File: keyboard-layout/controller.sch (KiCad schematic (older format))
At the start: 15 parts, among them J1 USB_mini_micro_B, SW1 SW_PUSH, X1 XTAL_GND

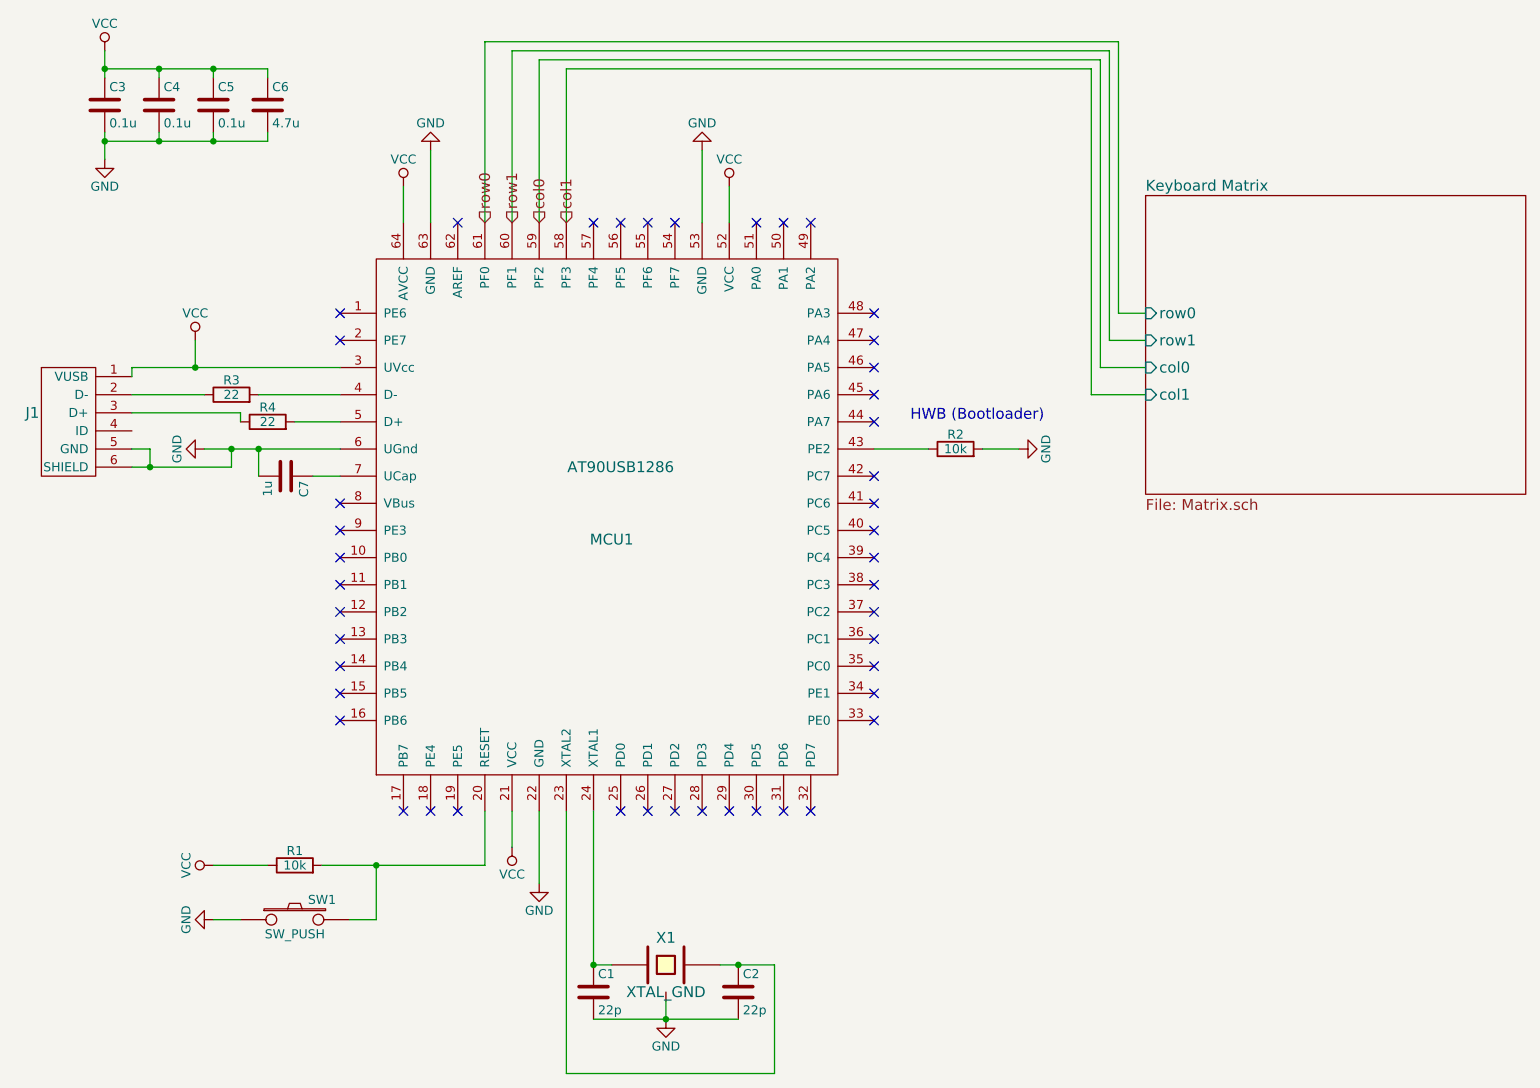
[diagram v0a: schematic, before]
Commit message: mx footprints
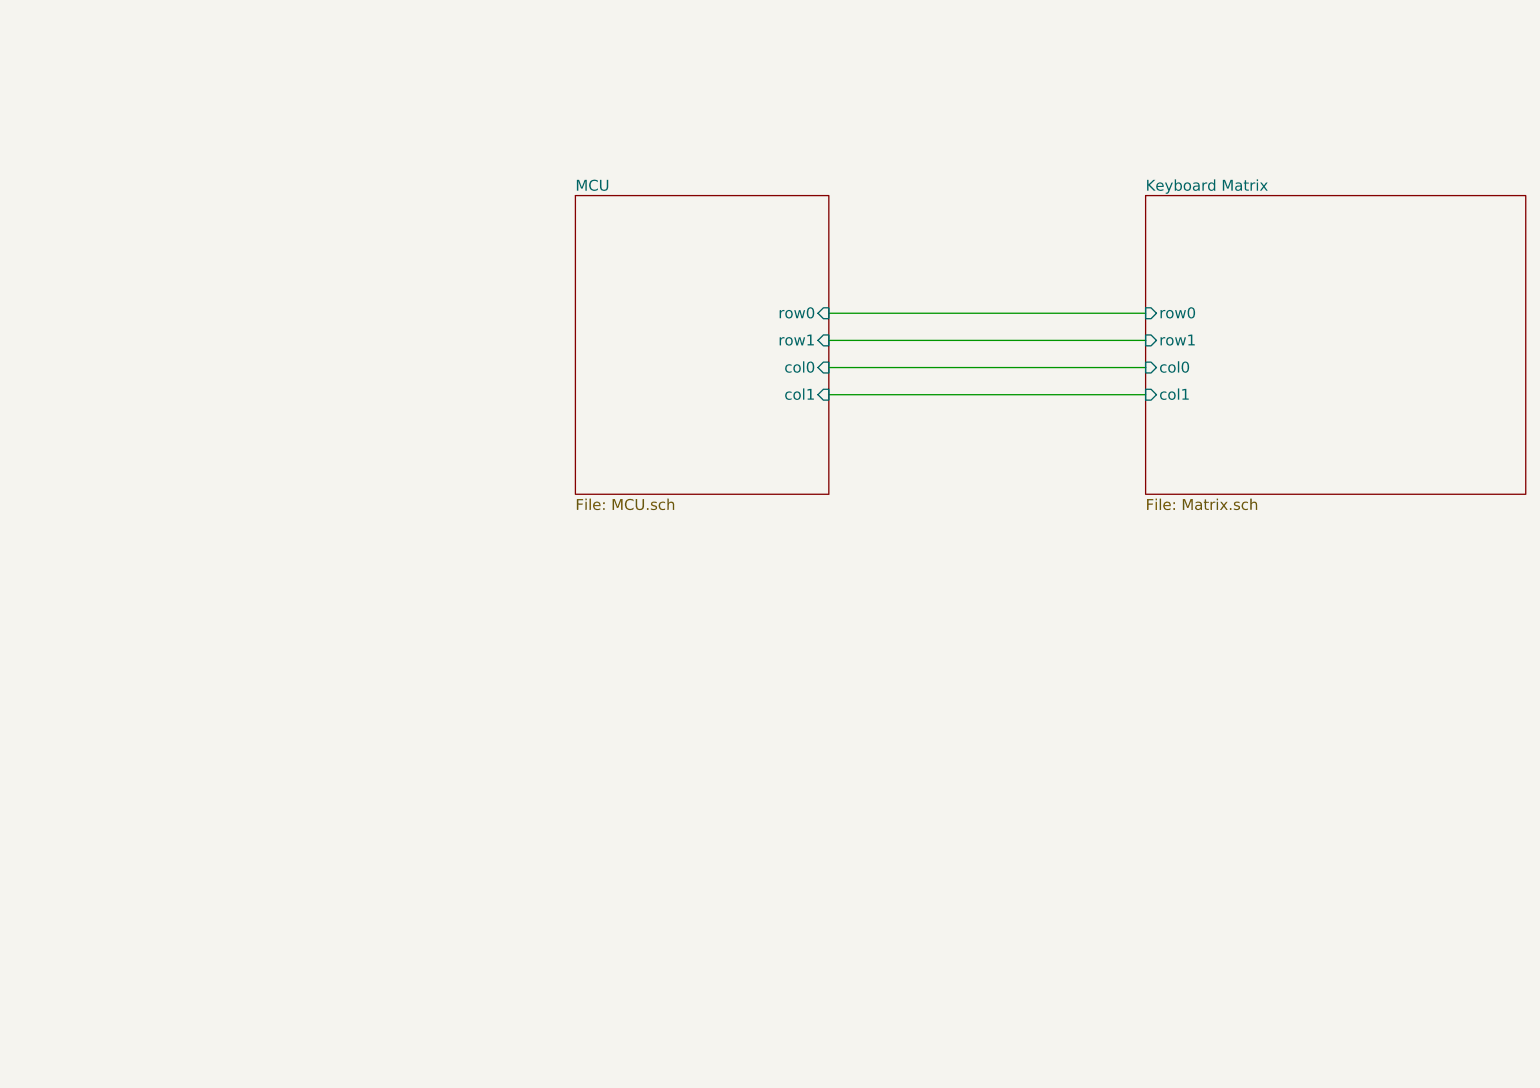
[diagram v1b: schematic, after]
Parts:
- removed C1, C2: 22p, Capacitors_SMD:C_0805_HandSoldering, symbol C
- removed C3, C4, C5: 0.1u, Capacitors_SMD:C_0805_HandSoldering, symbol C
- removed C6: 4.7u, Capacitors_SMD:C_0805_HandSoldering, symbol C
- removed C7: 1u, Capacitors_SMD:C_0805_HandSoldering, symbol C
- removed J1: USB_mini_micro_B, keyboard_parts:USB_miniB_hirose_5S8, symbol USB_mini_micro_B
- removed MCU1: AT90USB1286, AT90USB1286-AU:QFP80P1600X1600X120-64N, symbol AT90USB1286
- removed R1, R2: 10k, Resistors_SMD:R_0805_HandSoldering, symbol R
- removed R3, R4: 22, Resistors_SMD:R_0805_HandSoldering, symbol R
- removed SW1: SW_PUSH, Buttons_Switches_SMD:SW_SPST_TL3342, symbol SW_PUSH
- removed X1: XTAL_GND, Crystals:Crystal_SMD_SeikoEpson_FA238-4pin_3.2x2.5mm, symbol XTAL_GND
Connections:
- no-connect marks 45 -> 0
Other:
- note removed: "HWB (Bootloader)"

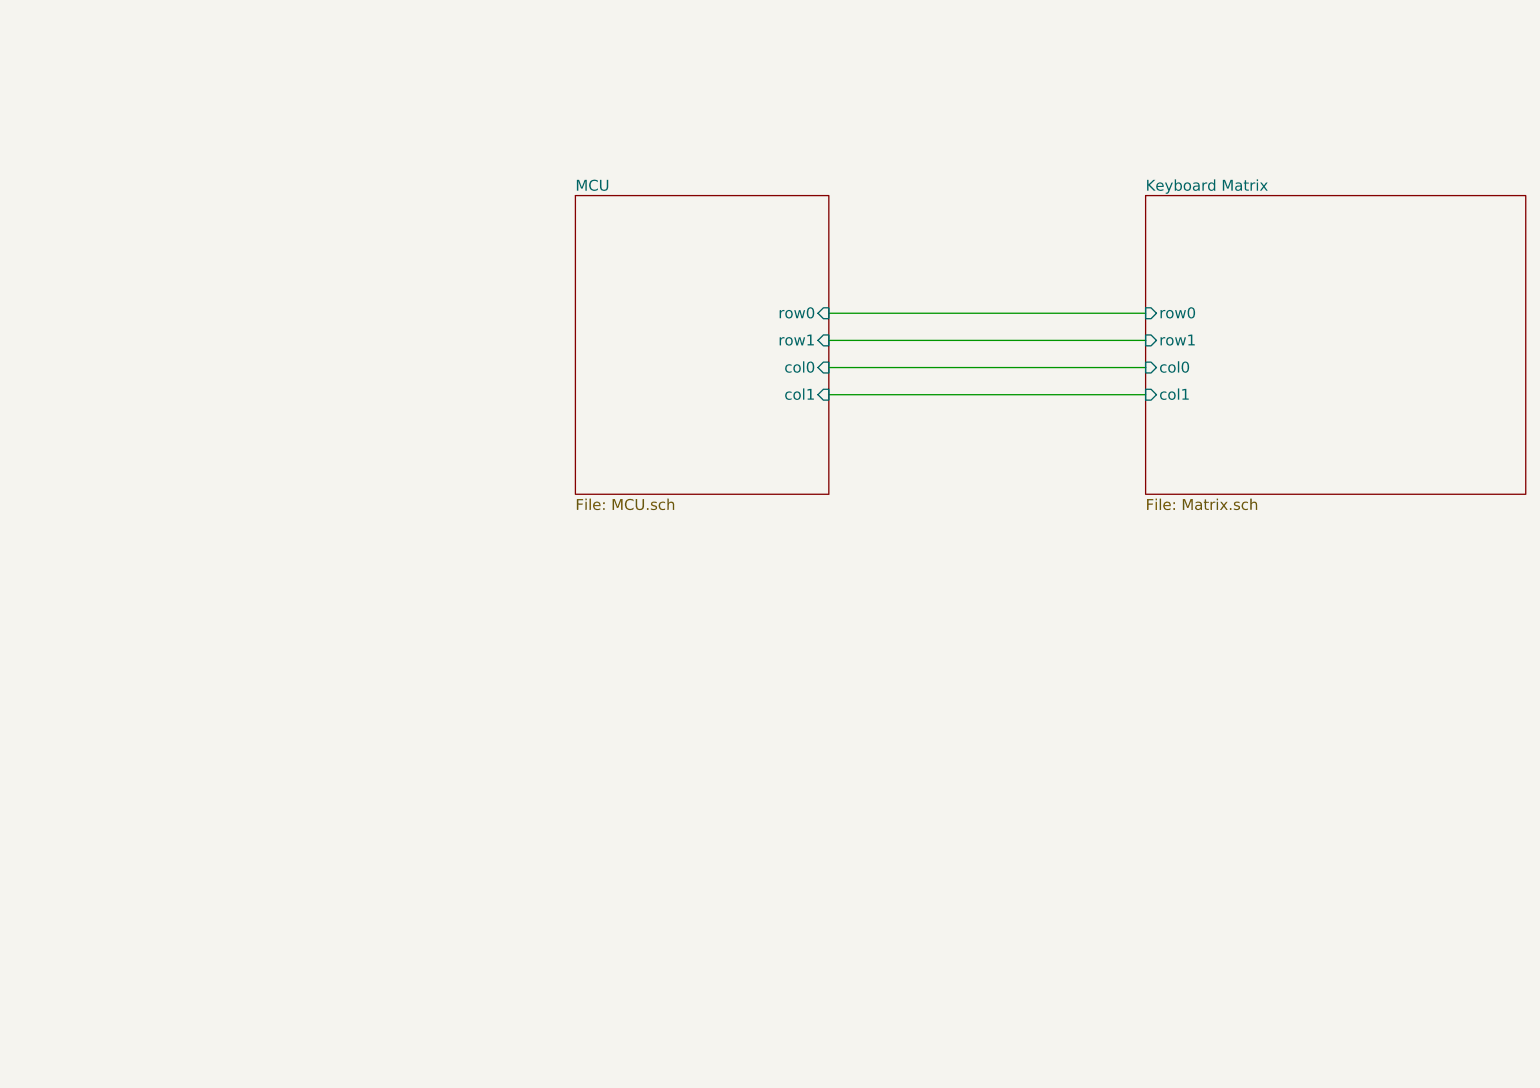
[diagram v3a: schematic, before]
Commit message: pcb progress
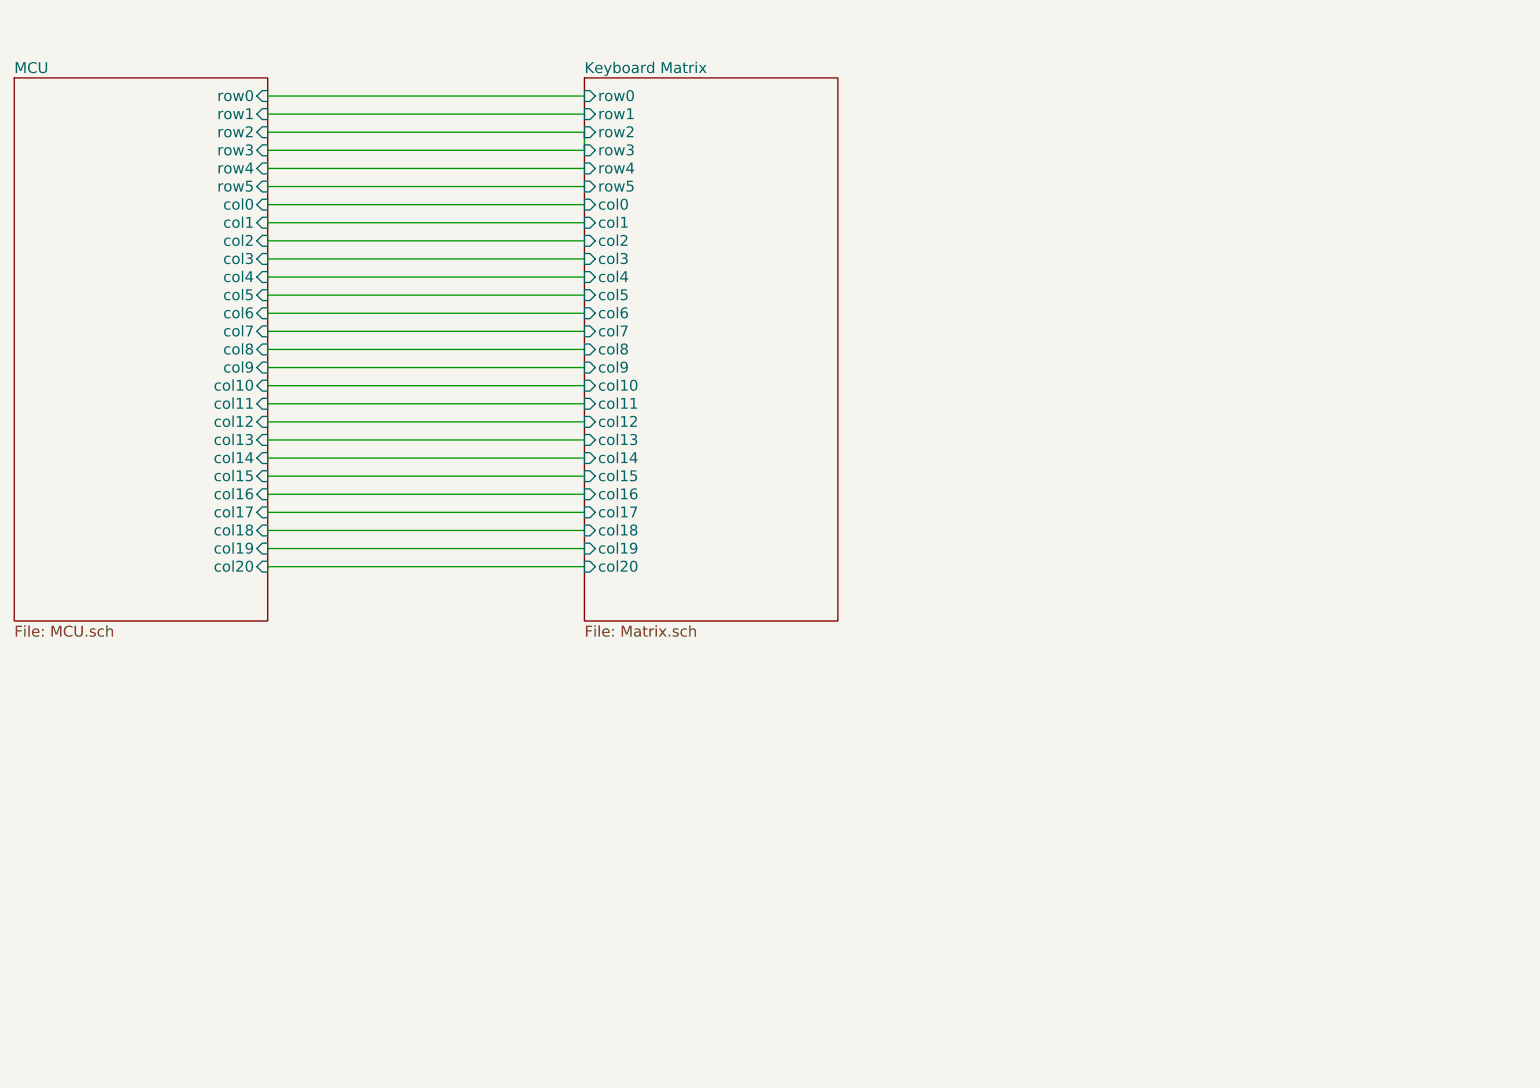
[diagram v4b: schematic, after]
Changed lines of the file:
@@
 $EndDescr
 $Sheet
-S 8100 2050 2100 1650
+S 5000 1400 1400 3000
 U 5AFAEA09
 F0 "Keyboard Matrix" 60
 F1 "Matrix.sch" 60
-F2 "col0" I L 8100 3000 60
-F3 "col1" I L 8100 3150 60
-F4 "row0" I L 8100 2700 60
-F5 "row1" I L 8100 2850 60
+F2 "row0" I L 5000 1500 60
+F3 "row1" I L 5000 1600 60
+F4 "col0" I L 5000 2100 60
+F5 "row2" I L 5000 1700 60
+F6 "row3" I L 5000 1800 60
+F7 "row4" I L 5000 1900 60
+F8 "row5" I L 5000 2000 60
+F9 "col1" I L 5000 2200 60
+F10 "col2" I L 5000 2300 60
+F11 "col3" I L 5000 2400 60
+F12 "col4" I L 5000 2500 60
+F13 "col5" I L 5000 2600 60
+F14 "col6" I L 5000 2700 60
+F15 "col7" I L 5000 2800 60
+F16 "col8" I L 5000 2900 60
+F17 "col9" I L 5000 3000 60
+F18 "col10" I L 5000 3100 60
+F19 "col11" I L 5000 3200 60
+F20 "col12" I L 5000 3300 60
+F21 "col13" I L 5000 3400 60
+F22 "col14" I L 5000 3500 60
+F23 "col15" I L 5000 3600 60
+F24 "col16" I L 5000 3700 60
+F25 "col17" I L 5000 3800 60
+F26 "col18" I L 5000 3900 60
+F27 "col19" I L 5000 4000 60
+F28 "col20" I L 5000 4100 60
 $EndSheet
+Wire Wire Line
+	3250 1500 5000 1500
+Wire Wire Line
+	5000 1600 3250 1600
 $Sheet
-S 4950 2050 1400 1650
+S 1850 1400 1400 3000
 U 5B003DFC
 F0 "MCU" 60
 F1 "MCU.sch" 60
-F2 "row0" I R 6350 2700 60
-F3 "row1" I R 6350 2850 60
-F4 "col0" I R 6350 3000 60
-F5 "col1" I R 6350 3150 60
+F2 "row0" I R 3250 1500 60
+F3 "row1" I R 3250 1600 60
+F4 "row2" I R 3250 1700 60
+F5 "row3" I R 3250 1800 60
+F6 "row4" I R 3250 1900 60
+F7 "row5" I R 3250 2000 60
+F8 "col0" I R 3250 2100 60
+F9 "col1" I R 3250 2200 60
+F10 "col2" I R 3250 2300 60
+F11 "col3" I R 3250 2400 60
+F12 "col4" I R 3250 2500 60
+F13 "col5" I R 3250 2600 60
+F14 "col6" I R 3250 2700 60
+F15 "col7" I R 3250 2800 60
+F16 "col8" I R 3250 2900 60
+F17 "col9" I R 3250 3000 60
+F18 "col10" I R 3250 3100 60
+F19 "col11" I R 3250 3200 60
+F20 "col12" I R 3250 3300 60
+F21 "col13" I R 3250 3400 60
+F22 "col14" I R 3250 3500 60
+F23 "col15" I R 3250 3600 60
+F24 "col16" I R 3250 3700 60
+F25 "col17" I R 3250 3800 60
+F26 "col18" I R 3250 3900 60
+F27 "col19" I R 3250 4000 60
+F28 "col20" I R 3250 4100 60
 $EndSheet
 Wire Wire Line
-	6350 2700 8100 2700
+	3250 1700 5000 1700
 Wire Wire Line
-	6350 2850 8100 2850
+	5000 1700 5000 1800
 Wire Wire Line
-	6350 3000 8100 3000
+	5000 1800 3250 1800
 Wire Wire Line
-	8100 3150 6350 3150
+	3250 1900 5000 1900
+Wire Wire Line
+	5000 2000 3250 2000
+Wire Wire Line
+	3250 2100 5000 2100
+Wire Wire Line
+	5000 2200 3250 2200
+Wire Wire Line
+	3250 2300 5000 2300
+Wire Wire Line
+	5000 2400 3250 2400
+Wire Wire Line
+	3250 2500 5000 2500
+Wire Wire Line
+	5000 2600 3250 2600
+Wire Wire Line
+	3250 2700 5000 2700
+Wire Wire Line
+	5000 2800 3250 2800
+Wire Wire Line
+	3250 2900 5000 2900
+Wire Wire Line
+	5000 3000 3250 3000
+Wire Wire Line
+	3250 3100 5000 3100
+Wire Wire Line
+	5000 3200 3250 3200
+Wire Wire Line
+	3250 3300 5000 3300
+Wire Wire Line
+	5000 3400 3250 3400
+Wire Wire Line
+	3250 3500 5000 3500
+Wire Wire Line
+	5000 3600 3250 3600
+Wire Wire Line
+	3250 3700 5000 3700
+Wire Wire Line
+	5000 3800 3250 3800
+Wire Wire Line
+	3250 3900 5000 3900
+Wire Wire Line
+	5000 4000 3250 4000
+Wire Wire Line
+	3250 4100 5000 4100
 $EndSCHEMATC
